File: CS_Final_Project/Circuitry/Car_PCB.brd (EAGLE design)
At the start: 43 x 34.7 mm, 28 parts, among them SW1 KMR2, SW2 KMR2, U1 SPX3819, U2 DRV8830, X1 ESP-12, X2 22-23-2021, X3 22-23-2021

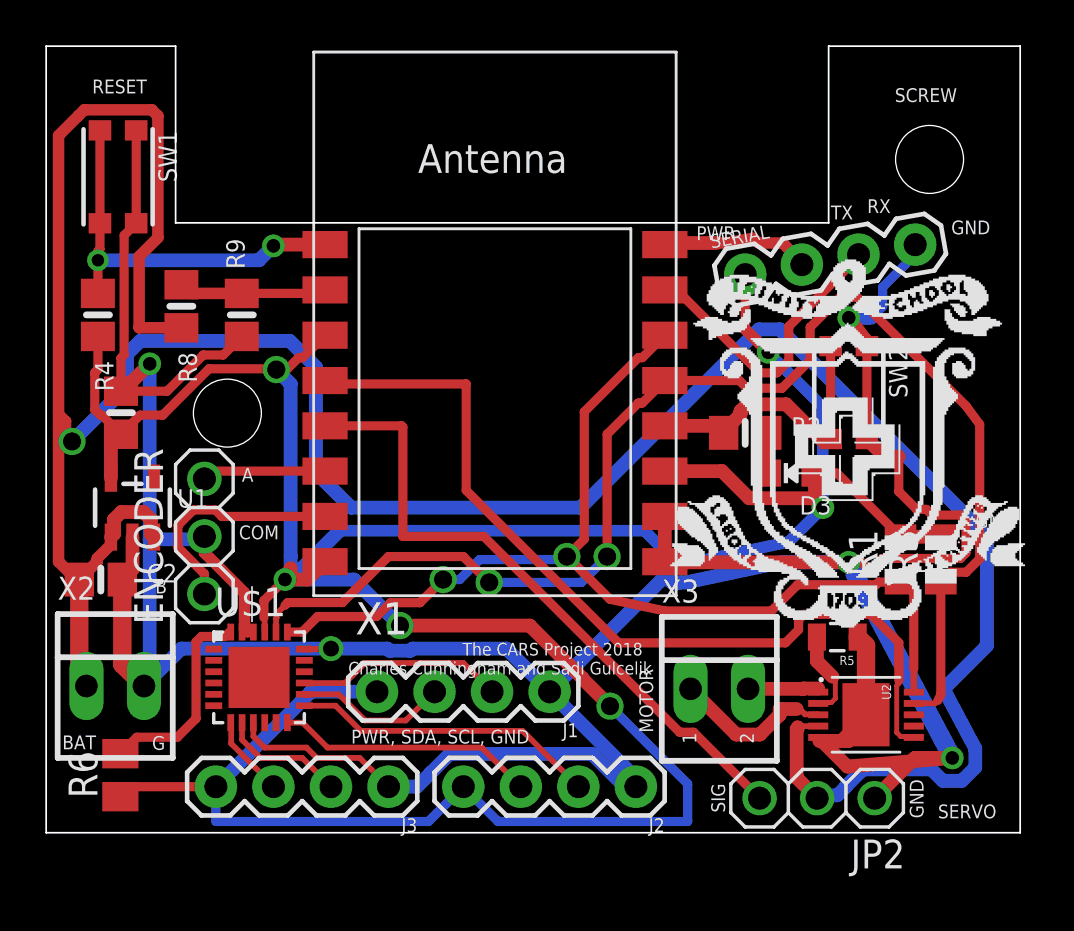
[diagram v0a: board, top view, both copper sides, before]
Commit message: Revert "Merge branch 'master' of https://github.com/mureytasroc/CarNetwork"
This reverts commit a45a0045a92c6dc43e66f74dc99afbd22e46fa88, reversing
changes made to 7d7a9c1b56f2fe83920f8a54f55361a334df6815.
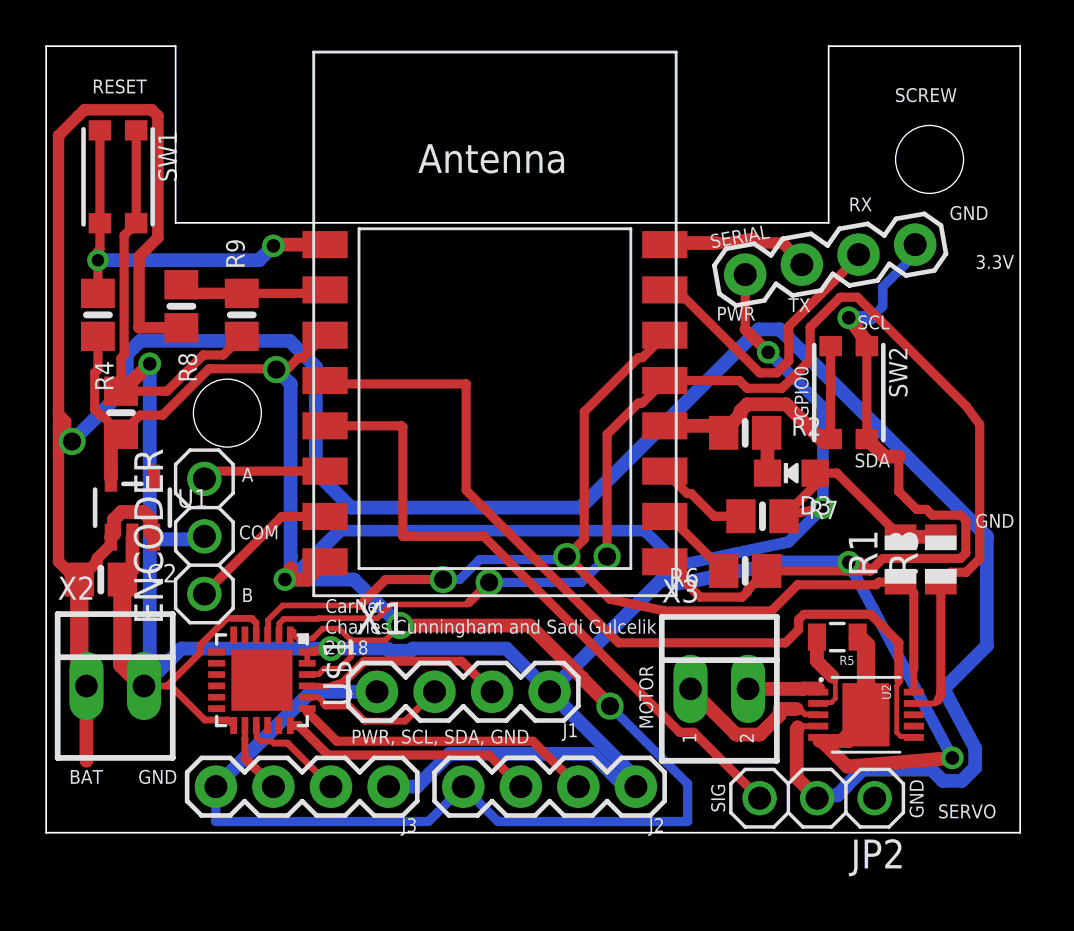
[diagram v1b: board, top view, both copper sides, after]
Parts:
- removed U$16: TRIN, OptoTher:TRIN
- added R7: 10K, microbuilder:0805-NO
- added U$13: (no value), microbuilder:PCBFEAT-REV-040
- R6: value 10k -> 10K; device adafruit:M0805 -> microbuilder:0805-NO
- moved R6 29.0 mm to (30.9, 10.0), turned to 180 degrees
- moved U$1 0.18 mm to (9.53, 5.21), turned to 270 degrees
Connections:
- removed net N$5: R6.2, U$1.24
- removed net SC4: U$1.11
- removed net SC5: J2.2, U$1.13
- removed net SC6: J1.2, U$1.15
- removed net SC7: U$1.17
- removed net SD4: U$1.10
- removed net SD5: J2.3, U$1.12
- removed net SD6: J1.3, U$1.14
- removed net SD7: U$1.16
- new net GPIO15: R6.2, X1.10
- new net GPIO2: R7.1, X1.11
- net 3.3V: now also R7.2, U$1.24, U$1.3; no longer R6.1, U$1.21, X1.11
- net GND: now also R6.1, U$1.1, U$1.12, U$1.2, U$1.21; no longer U$1.18, U$1.22, U$1.23, U$1.9, X1.10
- net SC0: now also J1.3, U$1.5; no longer U$1.2
- net SC1: now also J2.3, U$1.7; no longer U$1.4
- net SC2: now also U$1.9; no longer U$1.6
- net SC3: now also J3.3, U$1.11; no longer J3.2, U$1.8
- net SCL: now also U$1.22; no longer U$1.19
- net SD0: now also J1.2, U$1.4; no longer U$1.1
- net SD1: now also J2.2, U$1.6; no longer U$1.3
- net SD2: now also U$1.8; no longer U$1.5
- net SD3: now also J3.2, U$1.10; no longer J3.3, U$1.7
- net SDA: now also U$1.23; no longer U$1.20
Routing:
- net SC5: track 13.6 -> 0.00 mm
- net SD1: track 0.00 -> 13.4 mm
- net SD5: track 11.5 -> 0.00 mm
- net SC1: track 0.00 -> 11.2 mm
- net SC6: track 9.18 -> 0.00 mm
- net SD0: track 0.00 -> 9.11 mm
- net N$5: track 9.02 -> 0.00 mm
- net SD6: track 6.75 -> 0.00 mm
- net SC0: track 0.00 -> 6.67 mm
- net GND: track 175.2 -> 168.8 mm
- net GPIO2: track 0.00 -> 4.19 mm
- net 3.3V: track 148.4 -> 144.6 mm
- net GPIO13: track 10.4 -> 6.74 mm
- net GPIO15: track 0.00 -> 3.60 mm
- net VBAT: track 130.2 -> 133.5 mm
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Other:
- board text added: "3.3V"
- board text added: "CarNet Charles Cunningham and Sadi Gulcelik 2018"
- board text added: "Contains FCC ID 2ADUIESP-12"
- board text added: "ESP8266 WiFi 3.3V Logic Level To Bootload: hold down GPIO0 during reset"
- board text added: "GPIO0"
- board text added: "PWR, SCL, SDA, GND"
- board text added: "SCL"
- board text added: "SDA"
- board text added: "V+: 3.5-16VDC VBat: 3.5-16VDC RX,RST: 5V OK"
- board text removed: "G"
- board text removed: "PWR, SDA, SCL, GND"
- board text removed: "The CARS Project 2018 Charles Cunningham and Sadi Gulcelik"
